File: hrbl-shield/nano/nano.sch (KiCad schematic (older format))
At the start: 51 parts, among them P1 Digital, P2 Analog, P3 CONN_01X01, P4 CONN_01X01, P5 CONN_01X01, P6 CONN_01X01, U1 SFH6206-3T, U10 SFH6206-3T, U11 SFH6206-3T, U12 SFH6206-3T, U13 SFH6206-3T, U14 SFH6206-3T, U15 IFX27001TFV50ATMA1CT-ND, U16 SFH6206-3T, U2 SFH6206-3T, U3 SFH6206-3T, U4 SFH6206-3T, U5 SFH6206-3T, U6 SFH6206-3T, U7 SFH6206-3T, U8 SFH6206-3T, U9 SFH6206-3T, Y1_PLUG_SOCKET1 Conn_01x08, Y2_PLUG_SOCKET1 Conn_01x08

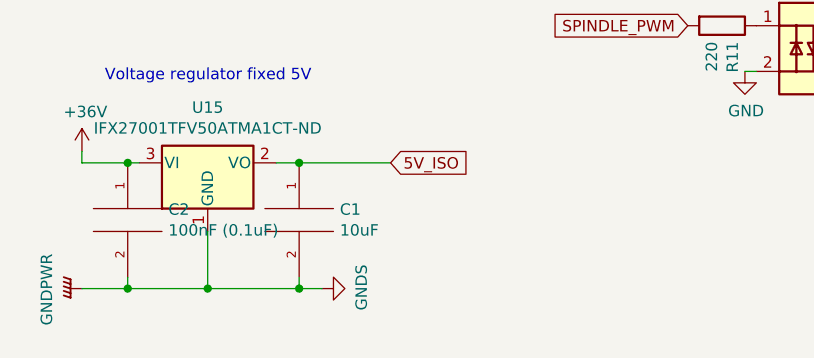
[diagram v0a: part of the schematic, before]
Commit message: updated Nano shield
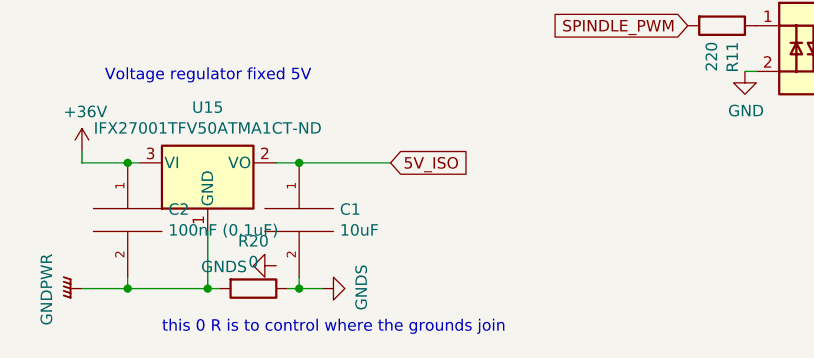
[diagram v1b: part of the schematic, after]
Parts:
- added R20: 0, Resistor_SMD:R_1206_3216Metric_Pad1.42x1.75mm_HandSolder, symbol Device:R
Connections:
- net GNDPWR: now also R20.2; no longer C1.2, PROBE1.1 (Pin_1), SPINDLE_CTR1.3 (Pin_3), U1.2, U1.3, U2.2, X_PLUG_SOCKET1.2 (Pin_2), X_PLUG_SOCKET1.4 (Pin_4), Y1_PLUG_SOCKET1.2 (Pin_2), Y1_PLUG_SOCKET1.4 (Pin_4), Y2_PLUG_SOCKET1.2 (Pin_2), Y2_PLUG_SOCKET1.4 (Pin_4), Z_PLUG_SOCKET1.2 (Pin_2), Z_PLUG_SOCKET1.4 (Pin_4)
- new net GNDS: C1.2, PROBE1.1 (Pin_1), R20.1, SPINDLE_CTR1.3 (Pin_3), U1.2, U1.3, U2.2, X_PLUG_SOCKET1.2 (Pin_2), X_PLUG_SOCKET1.4 (Pin_4), Y1_PLUG_SOCKET1.2 (Pin_2), Y1_PLUG_SOCKET1.4 (Pin_4), Y2_PLUG_SOCKET1.2 (Pin_2), Y2_PLUG_SOCKET1.4 (Pin_4), Z_PLUG_SOCKET1.2 (Pin_2), Z_PLUG_SOCKET1.4 (Pin_4)
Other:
- note added: "this 0 R is to control where the grounds join"
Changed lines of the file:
@@
 Text Label 1550 2350 0    50   ~ 0
 PWR_SIG
-Connection ~ 3750 7800
-Connection ~ 4150 7800
 $Comp
 L Device:R R16
@@
 Wire Wire Line
 	7100 3350 7250 3350
+$Comp
+L power:GNDS #PWR0114
+U 1 1 5B8A262D
+P 4050 7700
+F 0 "#PWR0114" H 4050 7450 50  0001 C CNN
+F 1 "GNDS" V 4055 7572 50  0000 R CNN
+F 2 "" H 4050 7700 50  0001 C CNN
+F 3 "" H 4050 7700 50  0001 C CNN
+	1    4050 7700
+	0    1    1    0
+$EndComp
+$Comp
+L Device:R R20
+U 1 1 5B8A2633
+P 3950 7800
+F 0 "R20" V 3743 7800 50  0000 C CNN
+F 1 "0" V 3834 7800 50  0000 C CNN
+F 2 "Resistor_SMD:R_1206_3216Metric_Pad1.42x1.75mm_HandSolder" V 3880 7800 50  0001 C CNN
+F 3 "~" H 3950 7800 50  0001 C CNN
+	1    3950 7800
+	0    1    1    0
+$EndComp
 Wire Wire Line
-	3750 7800 4150 7800
+	3800 7800 3750 7800
+Connection ~ 3750 7800
+Wire Wire Line
+	4100 7800 4150 7800
+Connection ~ 4150 7800
+Text Notes 3550 8000 0    50   ~ 0
+this 0 R is to control where the grounds join
 $EndSCHEMATC

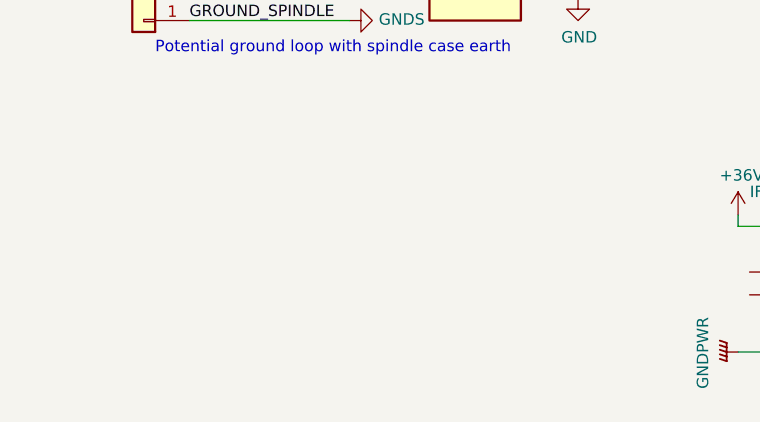
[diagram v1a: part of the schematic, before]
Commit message: Nano sheild
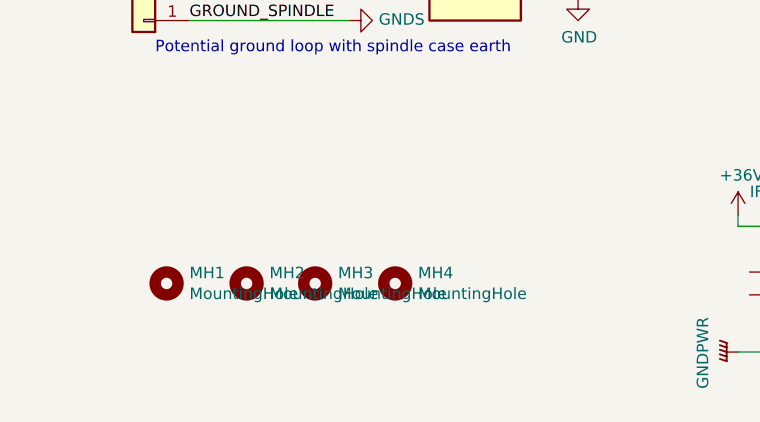
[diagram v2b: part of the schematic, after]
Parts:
- added MH1, MH2, MH3, MH4: MountingHole, MountingHole:MountingHole_4.5mm_Pad, symbol Mechanical:MountingHole
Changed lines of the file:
@@
 Text Notes 3550 8000 0    50   ~ 0
 this 0 R is to control where the grounds join
+$Comp
+L Mechanical:MountingHole MH4
+U 1 1 5B8B75FD
+P 1700 7500
+F 0 "MH4" H 1800 7546 50  0000 L CNN
+F 1 "MountingHole" H 1800 7455 50  0000 L CNN
+F 2 "MountingHole:MountingHole_4.5mm_Pad" H 1700 7500 50  0001 C CNN
+F 3 "~" H 1700 7500 50  0001 C CNN
+	1    1700 7500
+	1    0    0    -1
+$EndComp
+$Comp
+L Mechanical:MountingHole MH3
+U 1 1 5B8B7AAF
+P 1350 7500
+F 0 "MH3" H 1450 7546 50  0000 L CNN
+F 1 "MountingHole" H 1450 7455 50  0000 L CNN
+F 2 "MountingHole:MountingHole_4.5mm_Pad" H 1350 7500 50  0001 C CNN
+F 3 "~" H 1350 7500 50  0001 C CNN
+	1    1350 7500
+	1    0    0    -1
+$EndComp
+$Comp
+L Mechanical:MountingHole MH2
+U 1 1 5B8B7CFB
+P 1050 7500
+F 0 "MH2" H 1150 7546 50  0000 L CNN
+F 1 "MountingHole" H 1150 7455 50  0000 L CNN
+F 2 "MountingHole:MountingHole_4.5mm_Pad" H 1050 7500 50  0001 C CNN
+F 3 "~" H 1050 7500 50  0001 C CNN
+	1    1050 7500
+	1    0    0    -1
+$EndComp
+$Comp
+L Mechanical:MountingHole MH1
+U 1 1 5B8B7D84
+P 700 7500
+F 0 "MH1" H 800 7546 50  0000 L CNN
+F 1 "MountingHole" H 800 7455 50  0000 L CNN
+F 2 "MountingHole:MountingHole_4.5mm_Pad" H 700 7500 50  0001 C CNN
+F 3 "~" H 700 7500 50  0001 C CNN
+	1    700  7500
+	1    0    0    -1
+$EndComp
 $EndSCHEMATC
